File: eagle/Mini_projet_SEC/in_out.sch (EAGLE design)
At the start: 20 parts

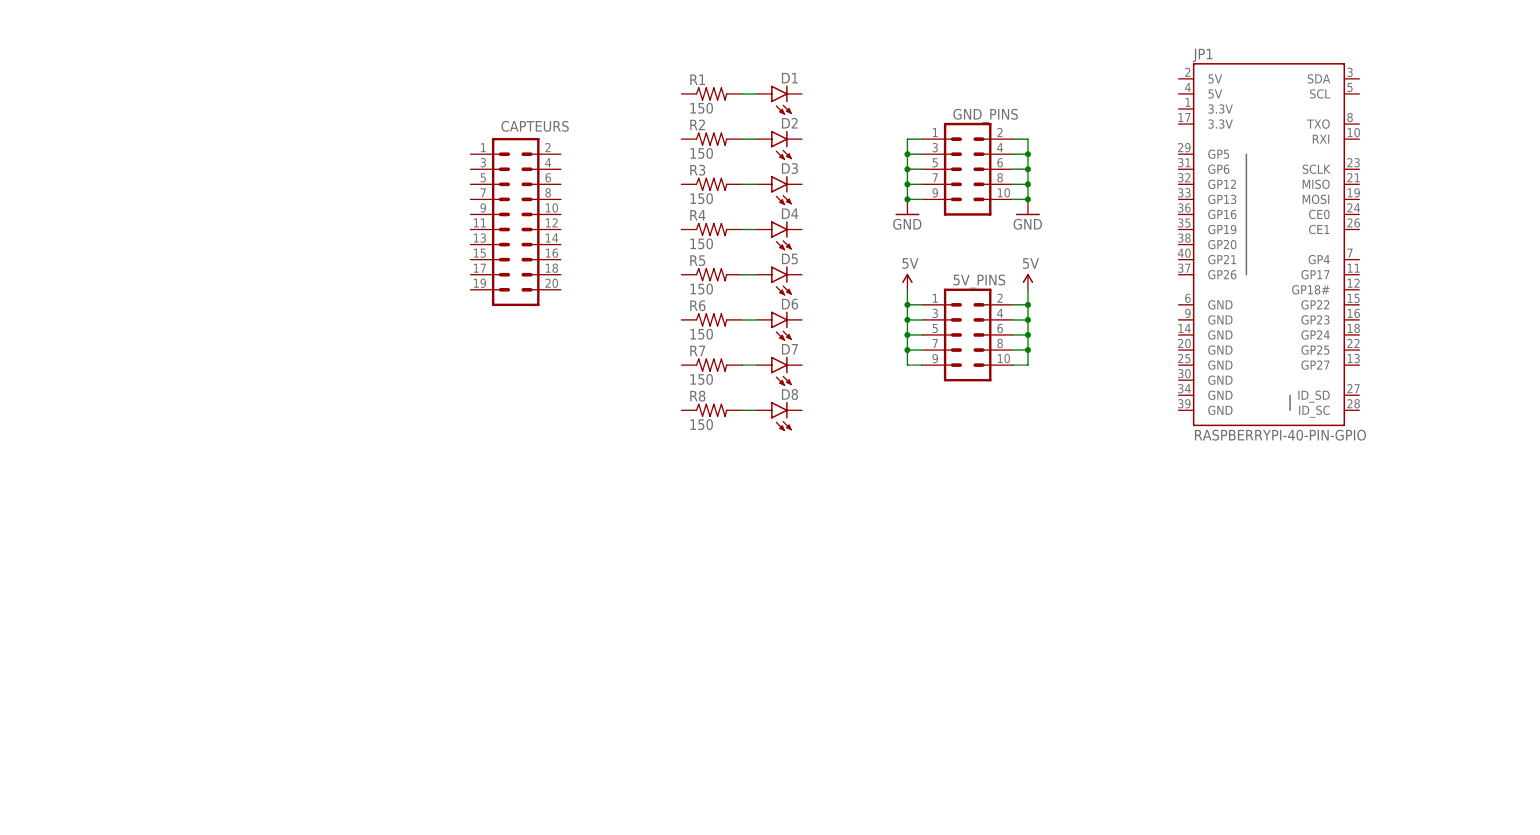
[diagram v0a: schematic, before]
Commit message: Update Eagle files. First usable PCB card base
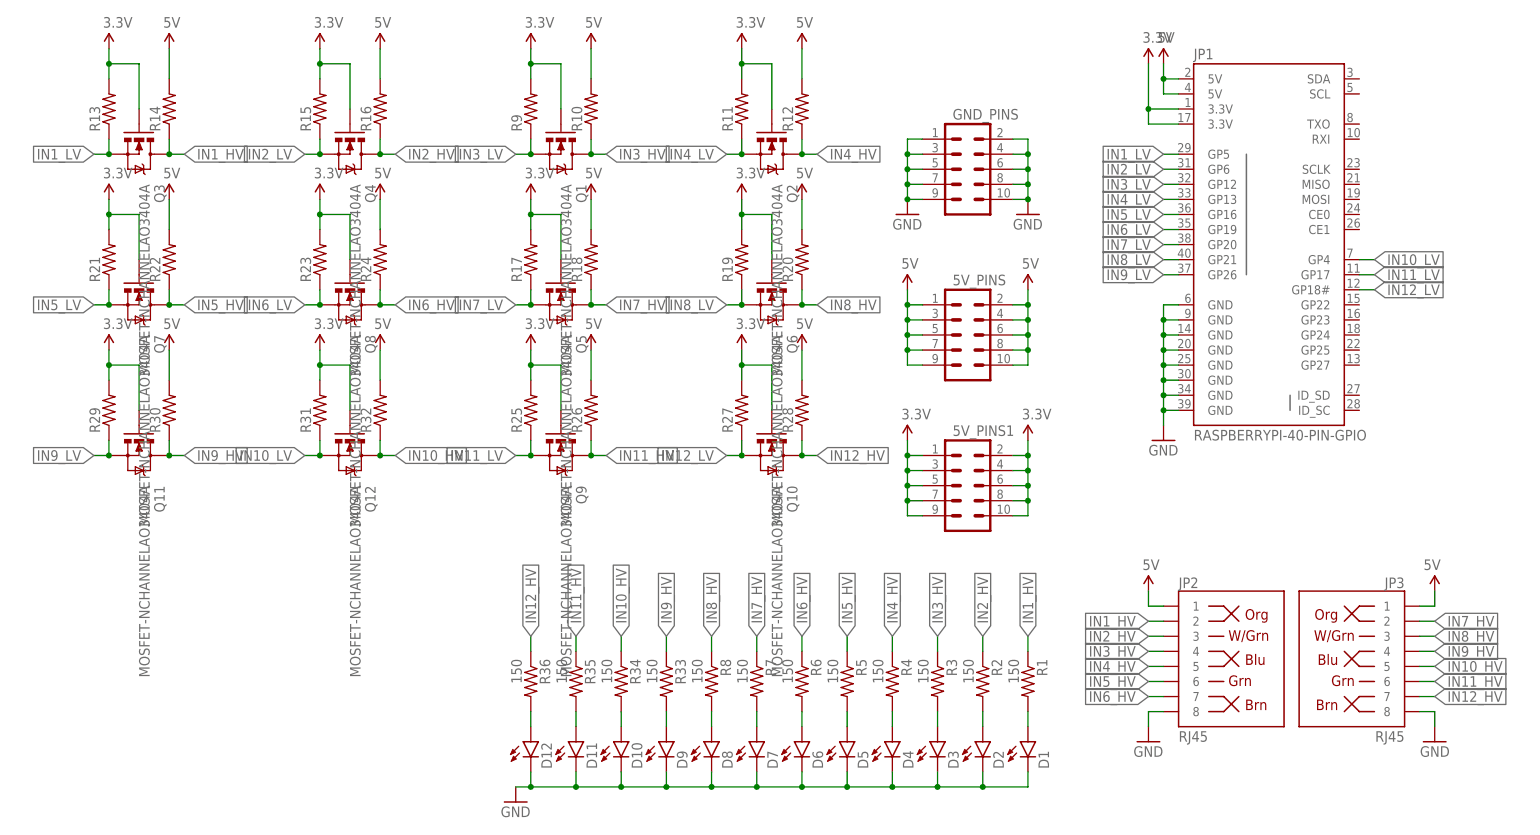
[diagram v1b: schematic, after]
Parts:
- removed CAPTEURS: (no value), SparkFun-Connectors:M10X22X10_LOCK
- added 5V_PINS1: (no value), SparkFun-Connectors:M05X2PTH
- added D10, D11, D12, D9: (no value), SparkFun-LED:LED5MM
- added JP2, JP3: RJ45, SparkFun-Connectors:RJ45-8PTH
- added Q1, Q10, Q11, Q12, Q2, Q3, Q4, Q5, Q6, Q7, Q8, Q9: MOSFET-NCHANNELAO3404A, SparkFun-DiscreteSemi:MOSFET-NCHANNELAO3404A
- added R10, R11, R12, R13, R14, R15, R16, R17, R18, R19, R20, R21, R22, R23, R24, R25, R26, R27, R28, R29, R30, R31, R32, R9: (no value), SparkFun-Passives:RESISTORPTH-1/4W
- added R33, R34, R35, R36: 150, SparkFun-Passives:RESISTOREZ
- 5V_PINS, GND_PINS: device SparkFun-Connectors:M05X2SHD_LOCK -> SparkFun-Connectors:M05X2PTH
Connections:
- new net 3.3V: 5V_PINS1.1, 5V_PINS1.10, 5V_PINS1.2, 5V_PINS1.3, 5V_PINS1.4, 5V_PINS1.5, 5V_PINS1.6, 5V_PINS1.7, 5V_PINS1.8, 5V_PINS1.9, JP1.3.3V@1, JP1.3.3V@17, Q1.G, Q10.G, Q11.G, Q12.G, Q2.G, Q3.G, Q4.G, Q5.G, Q6.G, Q7.G, Q8.G, Q9.G, R11.2, R13.2, R15.2, R17.2, R19.2, R21.2, R23.2, R25.2, R27.2, R29.2, R31.2, R9.2
- new net IN10_HV: JP3.5, Q12.D, R32.1, R34.1
- new net IN10_LV: JP1.GP4, Q12.S, R31.1
- new net IN11_HV: JP3.6, Q9.D, R26.1, R35.1
- new net IN11_LV: JP1.GP17, Q9.S, R25.1
- new net IN12_HV: JP3.7, Q10.D, R28.1, R36.1
- new net IN12_LV: JP1.GP18#, Q10.S, R27.1
- new net IN1_HV: JP2.2, Q3.D, R1.1, R14.1
- new net IN1_LV: JP1.GP5, Q3.S, R13.1
- new net IN2_HV: JP2.3, Q4.D, R16.1, R2.1
- new net IN2_LV: JP1.GP6, Q4.S, R15.1
- new net IN3_HV: JP2.4, Q1.D, R10.1, R3.1
- new net IN3_LV: JP1.GP12, Q1.S, R9.1
- new net IN4_HV: JP2.5, Q2.D, R12.1, R4.1
- new net IN4_LV: JP1.GP13, Q2.S, R11.1
- new net IN5_HV: JP2.6, Q7.D, R22.1, R5.1
- new net IN5_LV: JP1.GP16, Q7.S, R21.1
- new net IN6_HV: JP2.7, Q8.D, R24.1, R6.1
- new net IN6_LV: JP1.GP19, Q8.S, R23.1
- new net IN7_HV: JP3.2, Q5.D, R18.1, R7.1
- new net IN7_LV: JP1.GP20, Q5.S, R17.1
- new net IN8_HV: JP3.3, Q6.D, R20.1, R8.1
- new net IN8_LV: JP1.GP21, Q6.S, R19.1
- new net IN9_HV: JP3.4, Q11.D, R30.1, R33.1
- new net IN9_LV: JP1.GP26, Q11.S, R29.1
- new net N$1: D9.A, R33.2
- new net N$11: D11.A, R35.2
- new net N$12: D12.A, R36.2
- new net N$2: D10.A, R34.2
- net 5V: now also JP1.5V@2, JP1.5V@4, JP2.1, JP3.1, R10.2, R12.2, R14.2, R16.2, R18.2, R20.2, R22.2, R24.2, R26.2, R28.2, R30.2, R32.2
- net GND: now also D1.C, D10.C, D11.C, D12.C, D2.C, D3.C, D4.C, D5.C, D6.C, D7.C, D8.C, D9.C, JP1.GND@14, JP1.GND@20, JP1.GND@25, JP1.GND@30, JP1.GND@34, JP1.GND@39, JP1.GND@6, JP1.GND@9, JP2.8, JP3.8
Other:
- moved on the sheet: D1, D2, D3, D4, D5, D6, D7, D8, R1, R2, R3, R4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
